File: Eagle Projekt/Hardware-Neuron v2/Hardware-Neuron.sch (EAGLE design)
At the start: 124 parts, among them Q1 FDN360P, Q10 BSS123, Q11 BSS123, Q12 BSS123, Q13 BCX71SMD, Q14 BSS123, Q15 BSS123, Q16 BSS123, Q17 BSS123, Q18 BSS123, Q19 BSS123, Q2 FDN360P, Q20 BSS123, Q21 BSS123, Q22 BCX71SMD, Q23 BSS123, Q24 BSS123, Q25 BSS123, Q26 BCX71SMD, Q27 BSS123, Q28 BSS123, Q29 BSS123, Q3 FDN360P, Q30 BCX71SMD, Q31 BSS123, Q32 BSS123, Q33 BSS123, Q34 BCX71SMD, Q35 BSS123, Q36 BSS123, Q37 BSS123, Q38 BCX71SMD, Q39 BSS123, Q4 FDN360P, Q40 BSS123, Q41 BSS123, Q5 FDN360P, Q6 FDN360P, Q7 FDN360P, Q8 FDN360P, Q9 FDN360P, T1 BC846, T2 BC846, T3 BC846, T4 BC846, T5 BC846, T6 BC846, T7 BC846, T8 BC846

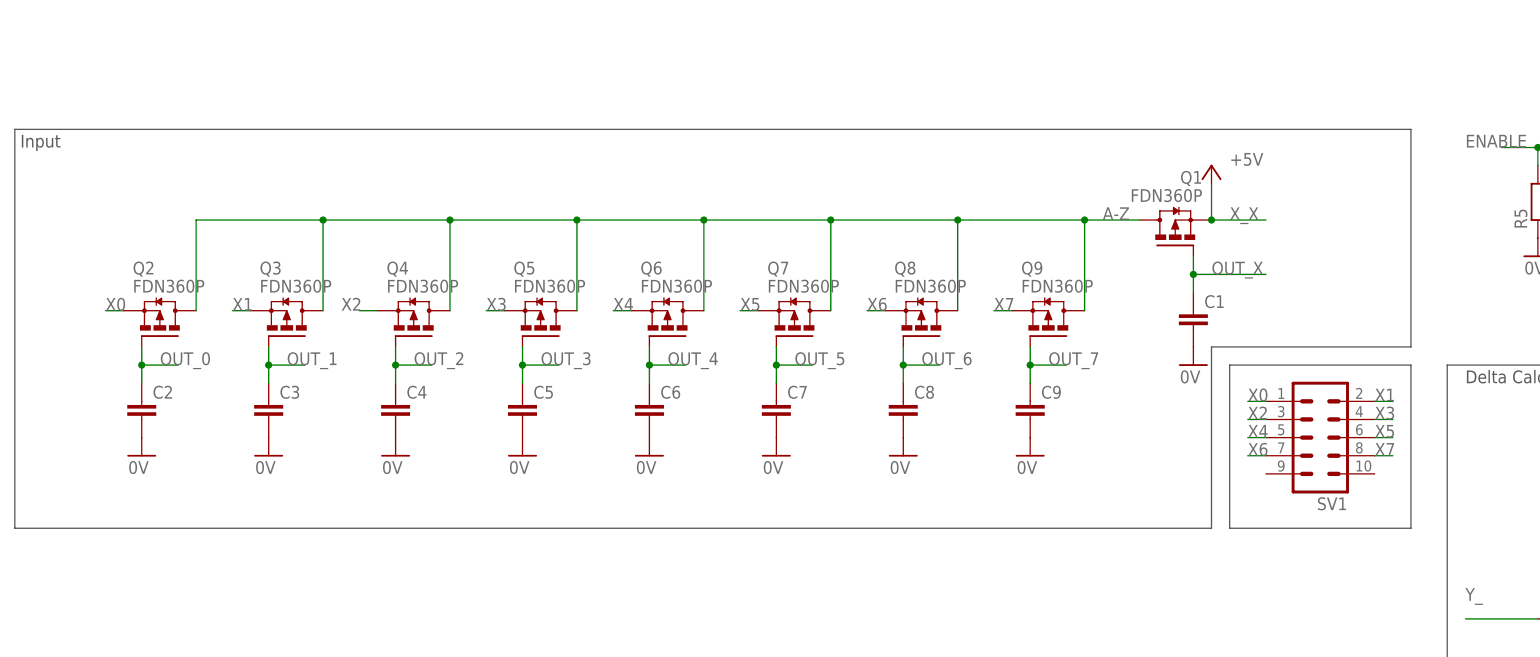
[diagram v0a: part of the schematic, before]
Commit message: Eagle Korrektur
(Nur oberflächlich)
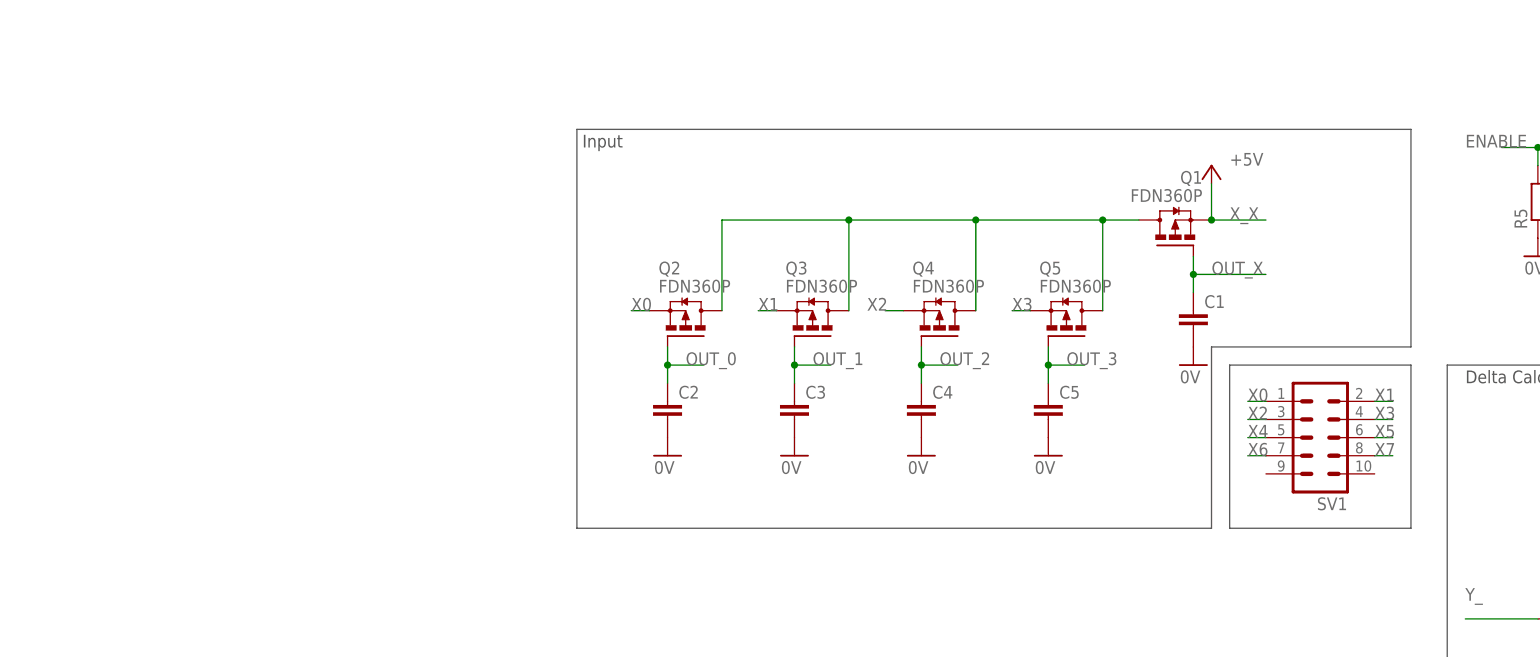
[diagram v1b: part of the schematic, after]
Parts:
- removed C6, C7, C8, C9: (no value), rcl:C-EUC1206
- removed Q6, Q7, Q8, Q9: FDN360P, transistor-power:FDN360P
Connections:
- removed net OUT_4: C6.1, Q6.G
- removed net OUT_5: C7.1, Q7.G
- removed net OUT_6: C8.1, Q8.G
- removed net OUT_7: C9.1, Q9.G
- net 0V: no longer C6.2, C7.2, C8.2, C9.2
- net A-Z: no longer Q6.D, Q7.D, Q8.D, Q9.D
- net X4: no longer Q6.S
- net X5: no longer Q7.S
- net X6: no longer Q8.S
- net X7: no longer Q9.S
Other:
- moved on the sheet: C2, C3, C4, C5, Q2, Q3, Q4, Q5
